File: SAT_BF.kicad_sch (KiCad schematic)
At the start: 15 parts, among them J1 Screw_Terminal_01x02, J2 Screw_Terminal_01x04, J3 Conn_02x10_Odd_Even, J4 Conn_02x20_Counter_Clockwise, U1 esp32-wemos-d1-mini, U2 ZC323200, U3 module_mpu6050, U4 HMC5883L, U7 INA219, U8 module_bme280, U9 esp32_38pins

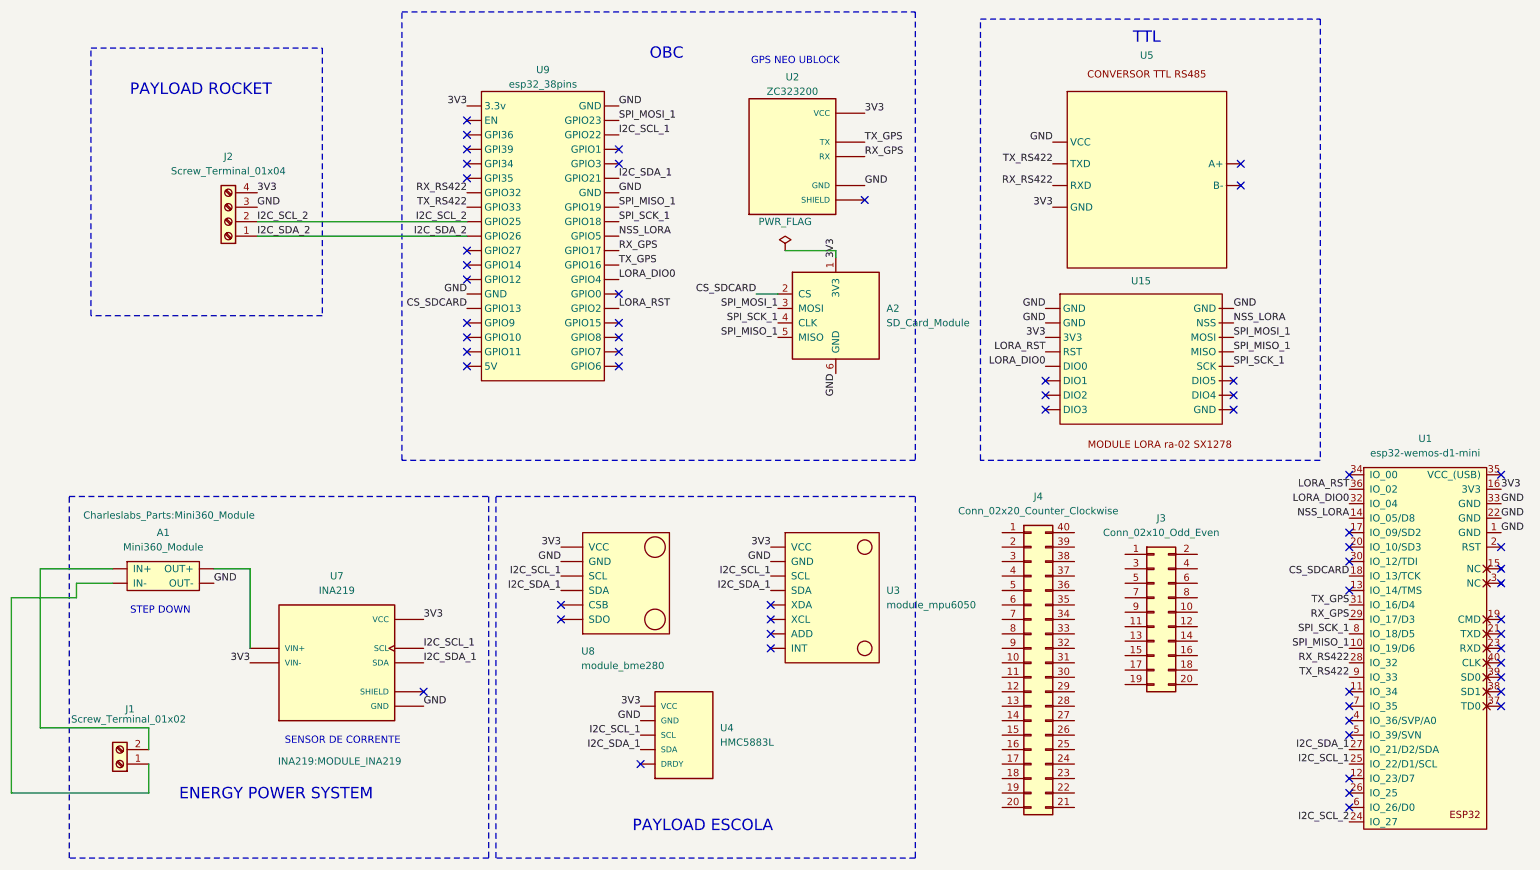
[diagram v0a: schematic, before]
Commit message: adicionando os barramentos
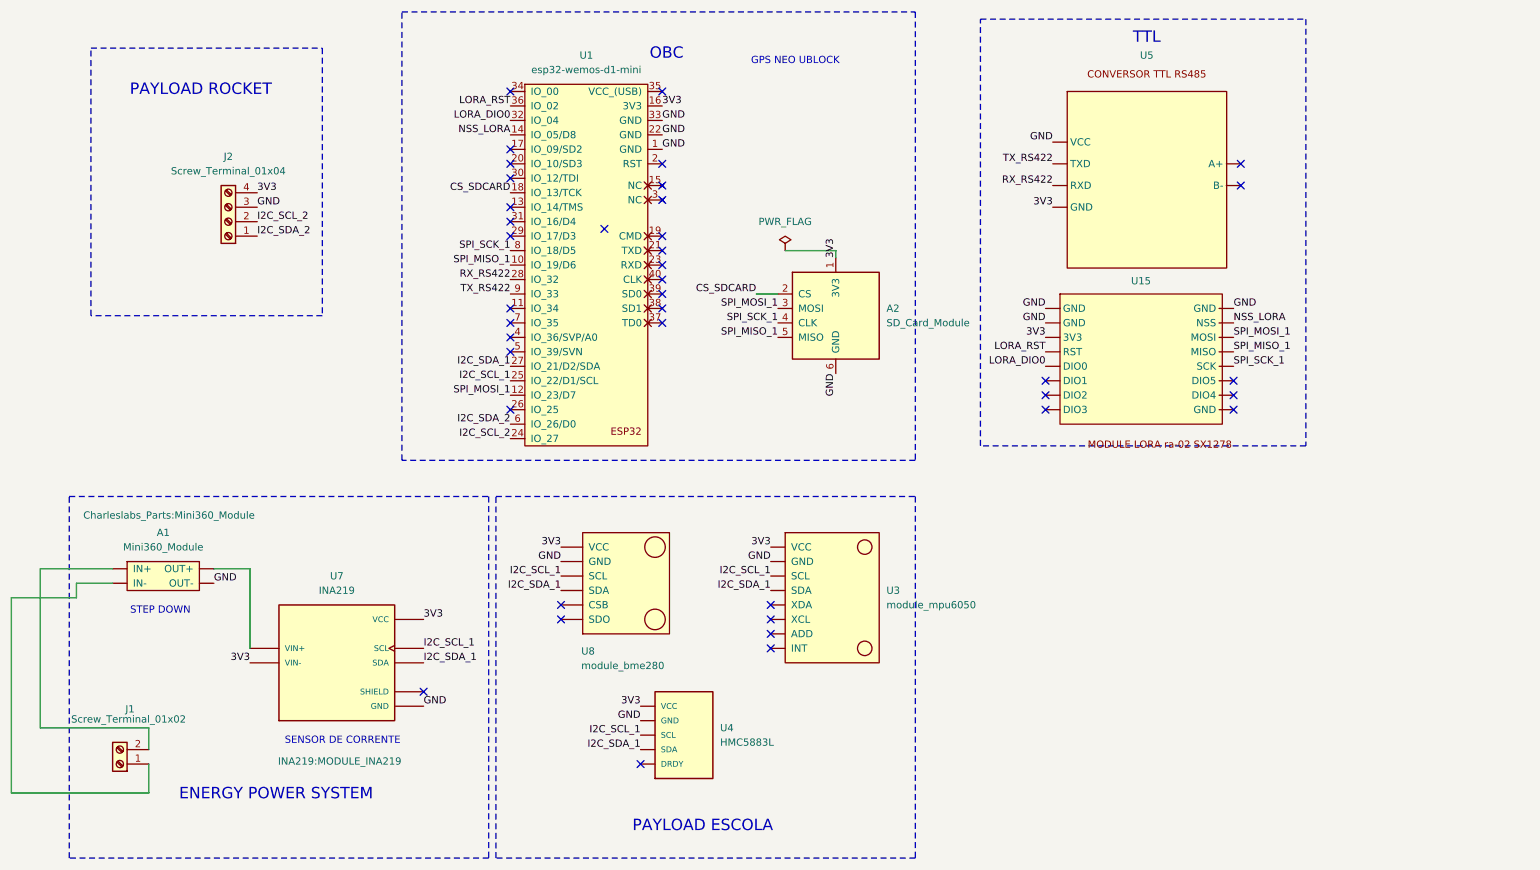
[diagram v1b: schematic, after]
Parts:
- removed J3: Conn_02x10_Odd_Even, Connector_PinHeader_2.54mm:PinHeader_2x10_P2.54mm_Vertical, symbol Connector_Generic:Conn_02x10_Odd_Even
- removed J4: Conn_02x20_Counter_Clockwise, symbol Connector_Generic:Conn_02x20_Counter_Clockwise
- removed U2: ZC323200, ZC323200:XCVR_ZC323200, symbol ZC323200:ZC323200
- removed U9: esp32_38pins, CTE_KICADMOD09_ESP32_38PIN:ESP-32_38PIN, symbol ESP32-38pin:Esp32
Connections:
- net I2C_SDA_2: now also U1.6 (IO_26/D0)
- net SPI_MOSI_1: now also U1.12 (IO_23/D7)
- net RX_GPS: no longer names the net of U1.29 (IO_17/D3)
- net TX_GPS: no longer names the net of U1.31 (IO_16/D4)
- no-connect marks 59 -> 40
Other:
- moved on the sheet: U1
